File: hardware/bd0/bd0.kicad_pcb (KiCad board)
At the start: 2 copper layers, 136.5 x 104 mm, 24 parts, among them J1 USB_C_Receptacle_USB2.0, J2 SJ-43514, U1 ATSAMD21G15B-A

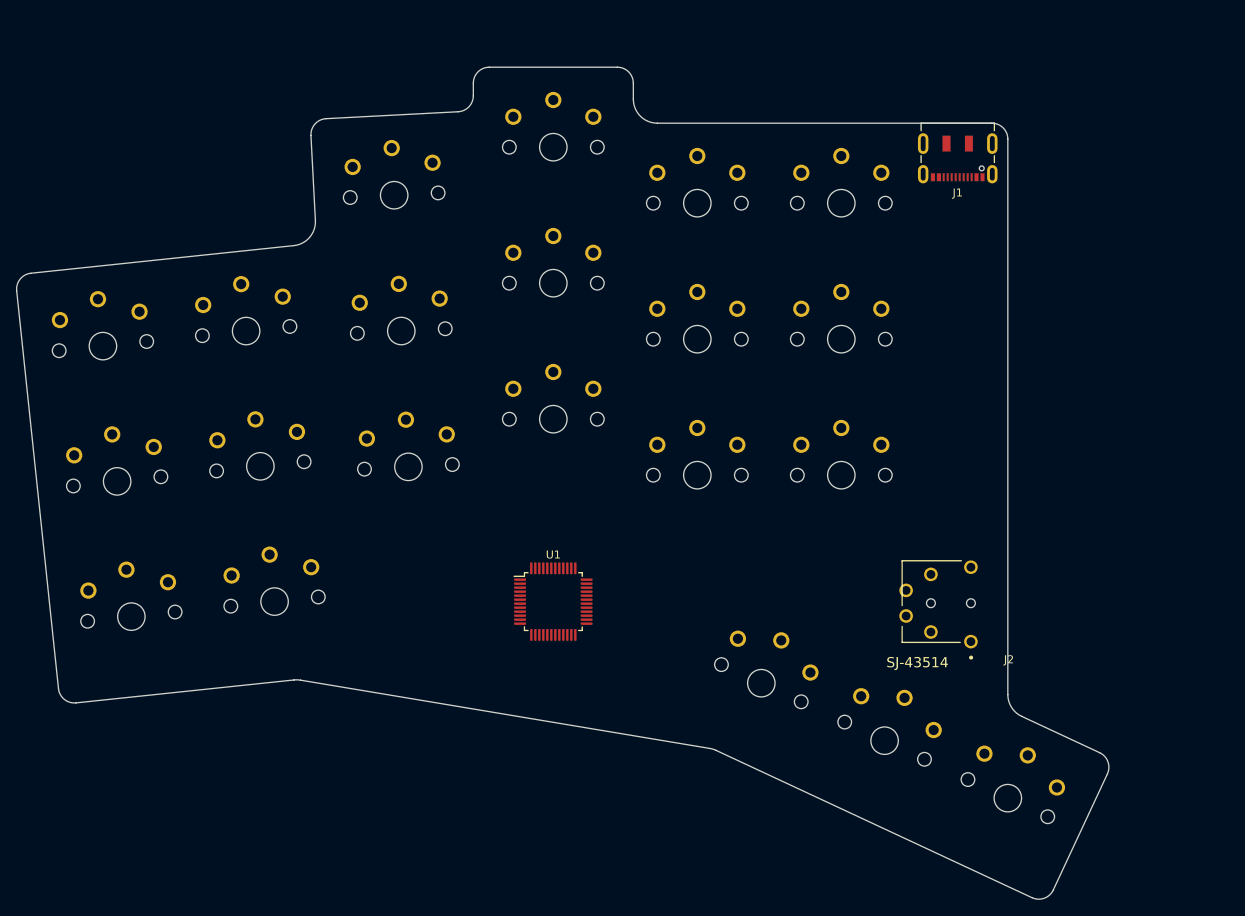
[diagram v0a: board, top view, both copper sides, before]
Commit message: Finished BD0 schematic and routing
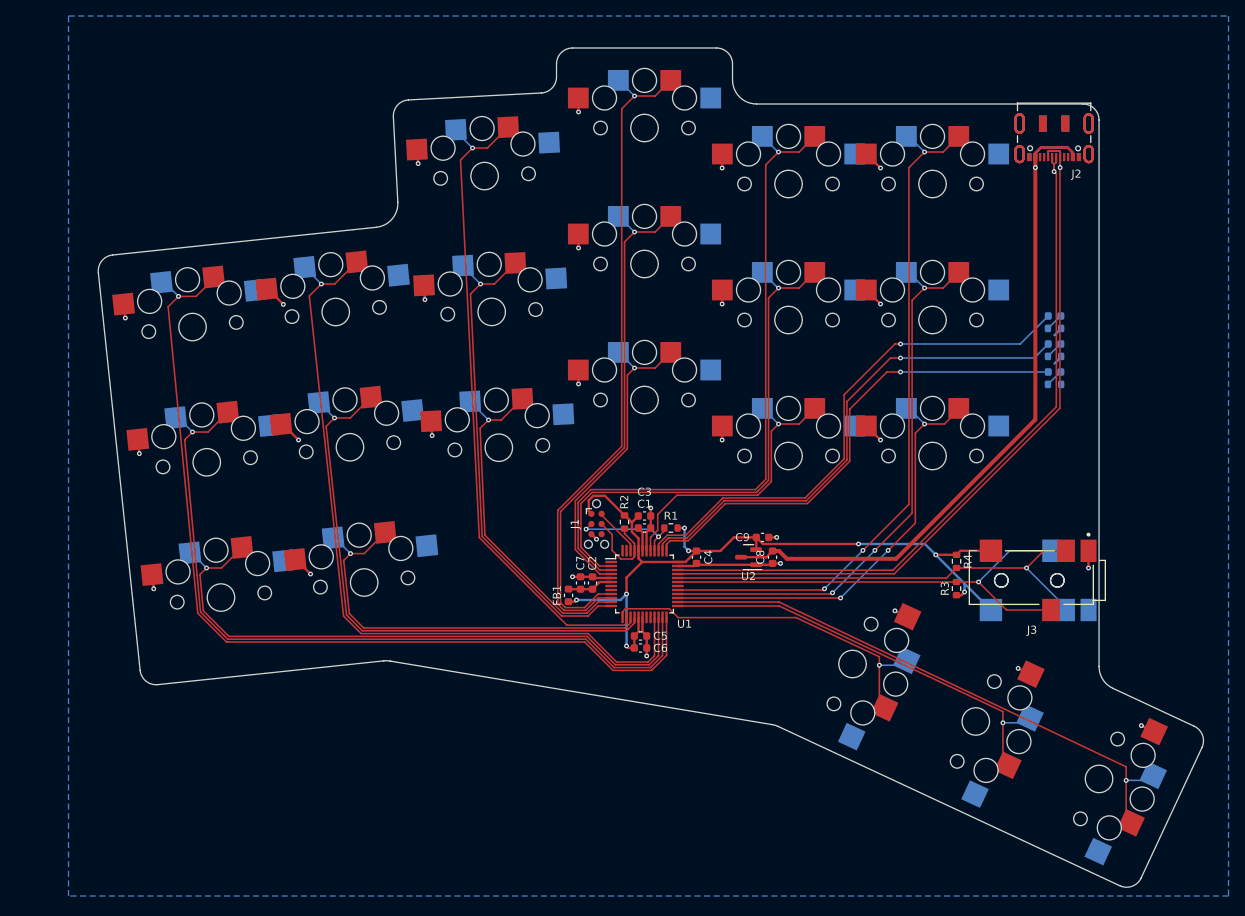
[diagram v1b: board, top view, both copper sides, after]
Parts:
- added C1: 1uF, Capacitor_SMD:C_0603_1608Metric, F.Cu at (222.0, 159.0)
- added C2: 0.1uF, Capacitor_SMD:C_0603_1608Metric, F.Cu at (215.5, 165.9)
- added C3: 0.1uF, Capacitor_SMD:C_0603_1608Metric, F.Cu at (222.0, 157.5)
- added C4: 0.1uF, Capacitor_SMD:C_0603_1608Metric, F.Cu at (228.5, 162.7)
- added C5: 0.1uF, Capacitor_SMD:C_0603_1608Metric, F.Cu at (221.5, 172.5)
- added C6: 10uF, Capacitor_SMD:C_0603_1608Metric, F.Cu at (221.5, 174.0)
- added C7: 10uF, Capacitor_SMD:C_0603_1608Metric, F.Cu at (214.0, 165.9)
- added C8: 1uF, Capacitor_SMD:C_0603_1608Metric, F.Cu at (238.0, 162.7)
- added C9: 1uF, Capacitor_SMD:C_0603_1608Metric, F.Cu at (236.8, 160.2)
- added D1: LED, Diode_SMD:D_0603_1608Metric, B.Cu at (273.2, 139.5)
- added D2: LED, Diode_SMD:D_0603_1608Metric, B.Cu at (273.2, 136.0)
- added D3: LED, Diode_SMD:D_0603_1608Metric, B.Cu at (273.2, 132.5)
- added FB1: FerriteBead, Inductor_SMD:L_0603_1608Metric, F.Cu at (212.5, 167.4)
- added J20: USB_C_Receptacle_USB2.0, Connector_USB:USB_C_Receptacle_JAE_DX07S016JA1R1500, B.Cu at (273.2, 109.6)
- added J3: SJ-43514, Conn_CUI_SJ-4351:CUI-SJ-43514-SMT-0, F.Cu at (271.1, 165.2)
- added J30: SJ-43514, Conn_CUI_SJ-4351:CUI-SJ-43514-SMT-0, B.Cu at (271.1, 165.9)
- added R1: 10k, Resistor_SMD:R_0603_1608Metric, F.Cu at (225.3, 159.0)
- added R2: 1k, Resistor_SMD:R_0603_1608Metric, F.Cu at (219.5, 158.2)
- added R3: 10k, Resistor_SMD:R_0603_1608Metric, F.Cu at (261.0, 166.6)
- added R4: 10k, Resistor_SMD:R_0603_1608Metric, F.Cu at (261.0, 163.2)
- added R5: 470, Resistor_SMD:R_0603_1608Metric, B.Cu at (273.2, 141.1)
- added R6: 470, Resistor_SMD:R_0603_1608Metric, B.Cu at (273.2, 137.6)
- added R7: 470, Resistor_SMD:R_0603_1608Metric, B.Cu at (273.2, 134.1)
- added U2: AP2127N-3.3, Package_TO_SOT_SMD:SOT-23, F.Cu at (235.0, 162.7)
- J1: value USB_C_Receptacle_USB2.0 -> Conn_02x03_Odd_Even; footprint Connector_USB:USB_C_Receptacle_JAE_DX07S016JA1R1500 -> Connector:Tag-Connect_TC2030-IDC-NL_2x03_P1.27mm_Vertical
- J2: value SJ-43514 -> USB_C_Receptacle_USB2.0; footprint Conn_CUI_SJ-4351:CUI-SJ-43514-0 -> Connector_USB:USB_C_Receptacle_JAE_DX07S016JA1R1500
- moved J1 64.7 mm to (216.0, 158.5), turned to -90 degrees
- moved J2 59.7 mm to (273.2, 109.6)
- moved S20 11.6 mm to (263.4, 183.2), turned to -115 degrees
- moved S10 11.6 mm to (222.0, 143.0)
- moved S11 11.6 mm to (222.0, 126.0)
- moved S12 11.6 mm to (222.0, 109.0)
- moved S13 11.6 mm to (240.0, 150.0)
- moved S14 11.6 mm to (240.0, 133.0)
- moved S15 11.6 mm to (240.0, 116.0)
- moved S16 11.6 mm to (258.0, 150.0)
- moved S17 11.6 mm to (258.0, 133.0)
- moved S18 11.6 mm to (258.0, 116.0)
- moved S19 11.6 mm to (248.0, 176.0), turned to -115 degrees
- moved S21 11.6 mm to (278.8, 190.4), turned to -115 degrees
- moved U1 11.6 mm to (222.0, 166.0)
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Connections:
- S1 pad 1: GND -> /outer_bottom
- S1 pad 2: /outer_bottom -> GND
- S10 pad 1: GND -> /middle_bottom
- S10 pad 2: /middle_bottom -> GND
- S11 pad 1: GND -> /middle_home
- S11 pad 2: /middle_home -> GND
- S12 pad 1: GND -> /middle_top
- S12 pad 2: /middle_top -> GND
- S13 pad 1: GND -> /index_bottom
- S13 pad 2: /index_bottom -> GND
- S14 pad 1: GND -> /index_home
- S14 pad 2: /index_home -> GND
- S15 pad 1: GND -> /index_top
- S15 pad 2: /index_top -> GND
- S16 pad 1: GND -> /inner_bottom
- S16 pad 2: /inner_bottom -> GND
- S17 pad 1: GND -> /inner_home
- S17 pad 2: /inner_home -> GND
- S18 pad 1: GND -> /inner_top
- S18 pad 2: /inner_top -> GND
- S19 pad 1: GND -> /near_thumb
- S19 pad 2: /near_thumb -> GND
- S2 pad 1: GND -> /outer_home
- S2 pad 2: /outer_home -> GND
- S20 pad 1: GND -> /home_thumb
- S20 pad 2: /home_thumb -> GND
- S21 pad 1: GND -> /far_thumb
- S21 pad 2: /far_thumb -> GND
- S3 pad 1: GND -> /outer_top
- S3 pad 2: /outer_top -> GND
- S4 pad 1: GND -> /pinky_bottom
- S4 pad 2: /pinky_bottom -> GND
- S5 pad 1: GND -> /pinky_home
- S5 pad 2: /pinky_home -> GND
- S6 pad 1: GND -> /pinky_top
- S6 pad 2: /pinky_top -> GND
- S7 pad 1: GND -> /ring_bottom
- S7 pad 2: /ring_bottom -> GND
- S8 pad 1: GND -> /ring_home
- S8 pad 2: /ring_home -> GND
- S9 pad 1: GND -> /ring_top
- S9 pad 2: /ring_top -> GND
- U1 pad 10: unconnected-(U1-Pad10) -> /middle_top
- U1 pad 11: unconnected-(U1-Pad11) -> /ring_bottom
- U1 pad 12: unconnected-(U1-Pad12) -> /ring_home
- U1 pad 13: /home_thumb -> /near_thumb
- U1 pad 14: unconnected-(U1-Pad14) -> /ring_top
- U1 pad 15: unconnected-(U1-Pad15) -> /pinky_bottom
- U1 pad 16: unconnected-(U1-Pad16) -> /pinky_home
- U1 pad 17: unconnected-(U1-Pad17) -> +3V3
- U1 pad 2: unconnected-(U1-Pad2) -> /index_home
- U1 pad 21: unconnected-(U1-Pad21) -> /pinky_top
- U1 pad 22: unconnected-(U1-Pad22) -> /outer_bottom
- U1 pad 23: unconnected-(U1-Pad23) -> /outer_home
- U1 pad 24: unconnected-(U1-Pad24) -> /outer_top
- U1 pad 25: unconnected-(U1-Pad25) -> /home_thumb
- U1 pad 26: unconnected-(U1-Pad26) -> /far_thumb
- U1 pad 27: unconnected-(U1-Pad27) -> /inner_bottom
- U1 pad 28: unconnected-(U1-Pad28) -> /inner_home
- U1 pad 29: unconnected-(U1-Pad29) -> /inner_top
- U1 pad 3: unconnected-(U1-Pad3) -> /index_top
- U1 pad 30: /RX -> unconnected-(U1-Pad30)
- U1 pad 31: /TX -> /SDA
- U1 pad 32: unconnected-(U1-Pad32) -> /SCL
- U1 pad 33: /USB_DM -> /USB_DN
- U1 pad 36: unconnected-(U1-Pad36) -> +3V3
- U1 pad 37: unconnected-(U1-Pad37) -> /LED0
- U1 pad 38: unconnected-(U1-Pad38) -> /LED1
- U1 pad 39: unconnected-(U1-Pad39) -> /LED2
- U1 pad 4: unconnected-(U1-Pad4) -> /middle_bottom
- U1 pad 40: unconnected-(U1-Pad40) -> /RESETn
- U1 pad 41: unconnected-(U1-Pad41) -> /index_bottom
- U1 pad 43: unconnected-(U1-Pad43) -> +1V2
- U1 pad 44: unconnected-(U1-Pad44) -> +3V3
- U1 pad 45: unconnected-(U1-Pad45) -> /SWCLK
- U1 pad 46: unconnected-(U1-Pad46) -> /SWDIO
- U1 pad 6: unconnected-(U1-Pad6) -> /3V3A
- U1 pad 9: unconnected-(U1-Pad9) -> /middle_home
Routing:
- net /outer_top: track 0.00 -> 115.9 mm, vias 0 -> 1
- net +3V3: track 0.00 -> 104.3 mm, vias 0 -> 8
- net /outer_home: track 0.00 -> 97.3 mm, vias 0 -> 1
- net /pinky_top: track 0.00 -> 97.2 mm, vias 0 -> 1
- net /USB_DN: track 0.00 -> 95.1 mm, vias 0 -> 1
- net +5V: track 0.00 -> 91.4 mm, vias 0 -> 1
- net /USB_DP: track 0.00 -> 91.1 mm, vias 0 -> 1
- net /inner_top: track 0.00 -> 86.5 mm, vias 0 -> 3
- net /index_top: track 0.00 -> 85.4 mm, vias 0 -> 1
- net /middle_top: track 0.00 -> 83.3 mm, vias 0 -> 1
- net /ring_top: track 0.00 -> 81.8 mm, vias 0 -> 1
- net GND: track 0.00 -> 79.4 mm, vias 0 -> 28
- net /outer_bottom: track 0.00 -> 79.0 mm, vias 0 -> 1
- net /far_thumb: track 0.00 -> 71.6 mm, vias 0 -> 1
- net /pinky_home: track 0.00 -> 71.5 mm, vias 0 -> 1
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- added copper zone on B.Cu, net GND
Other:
- board size 136.5 x 104 mm -> 138.2 x 104.9 mm
